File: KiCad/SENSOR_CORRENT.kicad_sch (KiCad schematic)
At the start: 4 parts, among them J1 Conn_01x08_Pin, SW1 SS-1GL2-F-D

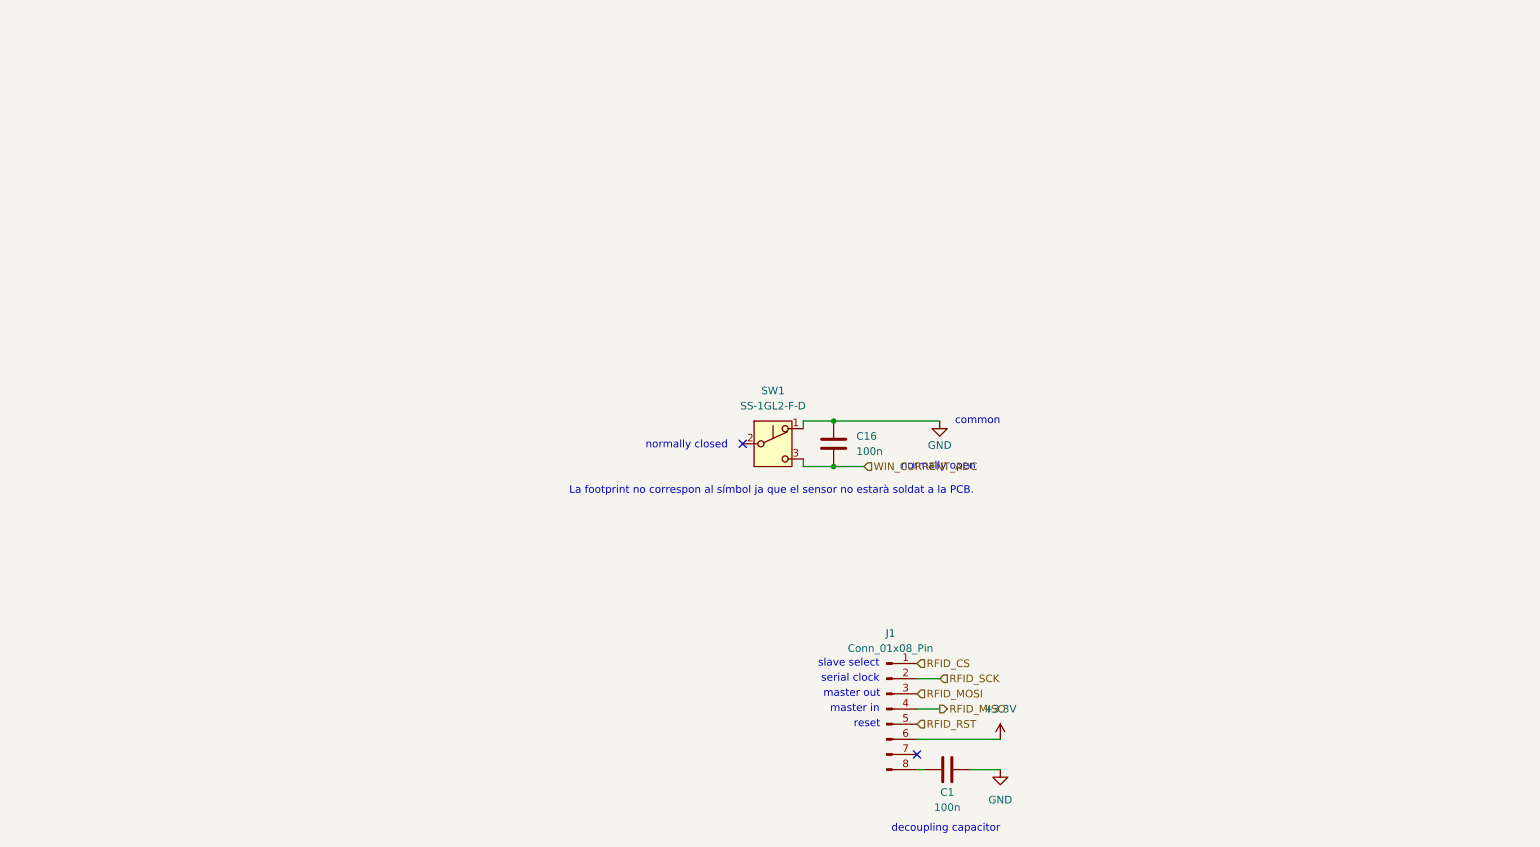
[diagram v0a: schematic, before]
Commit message: Versió final de l'esquematic
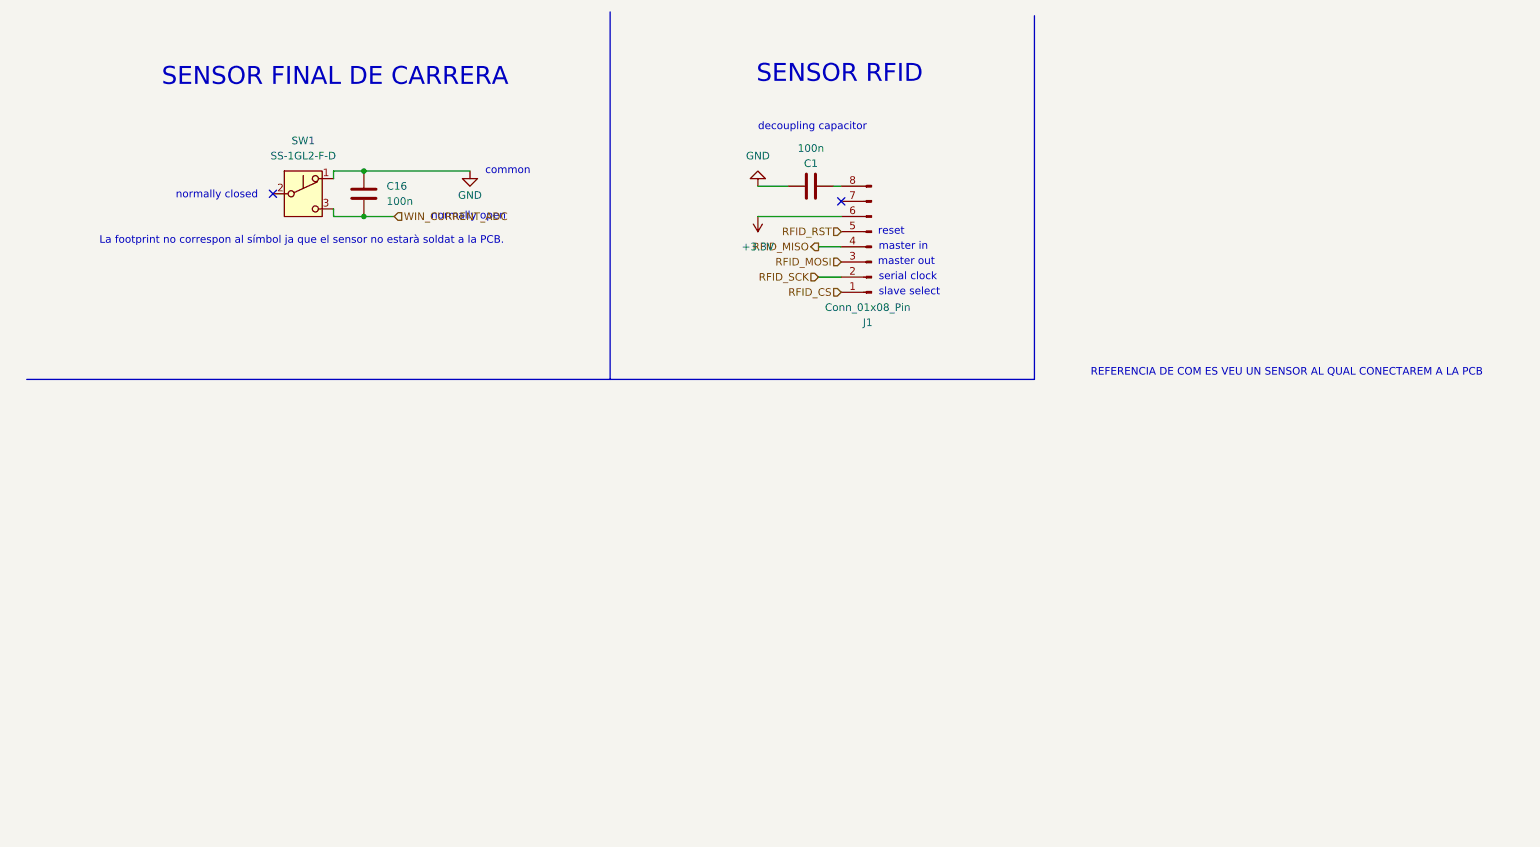
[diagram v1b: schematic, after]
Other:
- note added: "REFERENCIA DE COM ES VEU UN SENSOR AL QUAL CONECTAREM A LA PCB"
- note added: "SENSOR FINAL DE CARRERA"
- note added: "SENSOR RFID"
- moved on the sheet: C1, C16, J1, SW1
